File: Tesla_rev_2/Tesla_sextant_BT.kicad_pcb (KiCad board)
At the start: 4 copper layers, 100 x 100 mm, 121 parts, among them J1 Conn_01x05, J2 Conn_01x02, J3 Conn_01x05, J4 Conn_01x02, J6 USB_C_Receptacle_USB2.0_16P, J7 Conn_01x03, J8 Conn_01x02, J9 Conn_01x02, K1 G5V-1, Q1 BC817, U1 ESP32-C3-WROOM-02, U2 PCM5102A, U4 TPA0211, U5 USBLC6-2SC6, U6 AP63203WU, U7 LD1117STR, U8 AD831, Y1 OSC25M-3.3I/S5

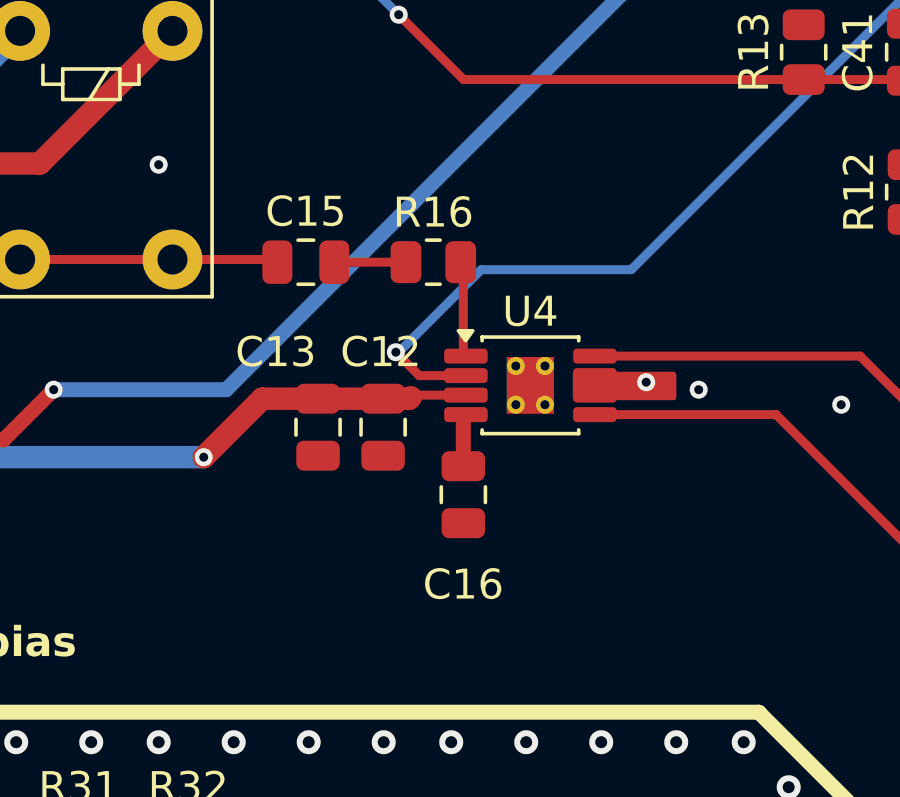
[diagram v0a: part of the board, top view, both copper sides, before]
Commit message: Final Project Commit
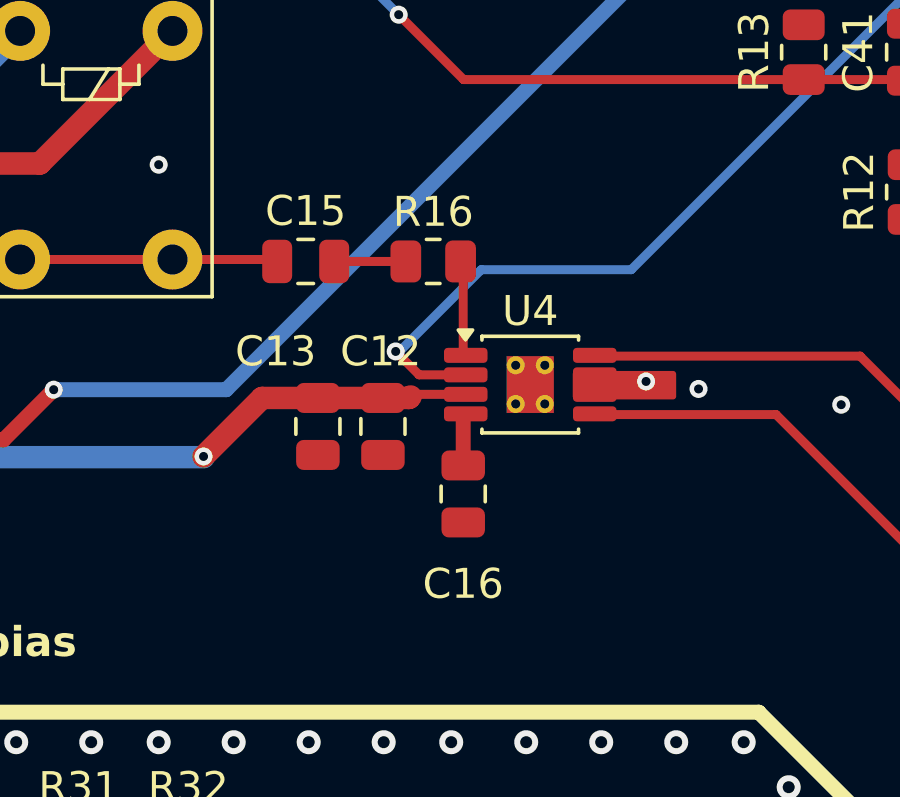
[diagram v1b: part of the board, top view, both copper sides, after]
